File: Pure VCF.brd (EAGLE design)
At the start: 33.6 x 100 mm, 82 parts, among them T1 TRANS_PAIR_PNP, U1 QUAD_OPAMP, U2 LM13700, U3 DUAL_OPAMP, U4 LM13700

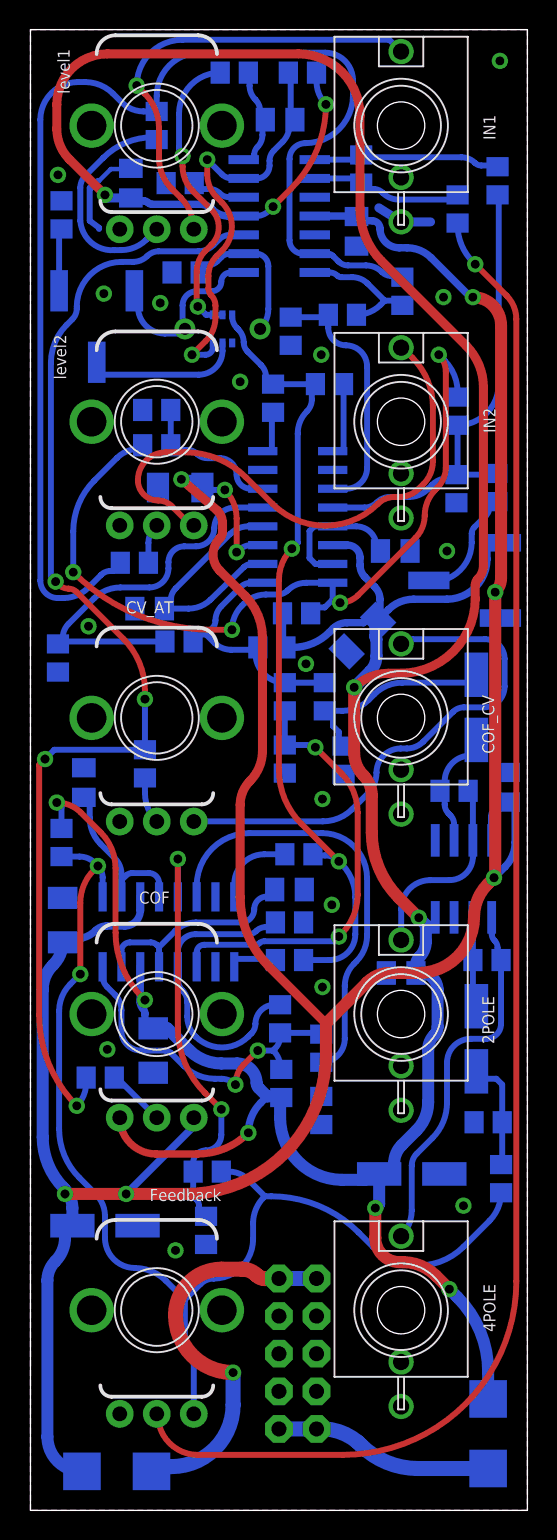
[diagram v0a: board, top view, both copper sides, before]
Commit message: VCF 2.2
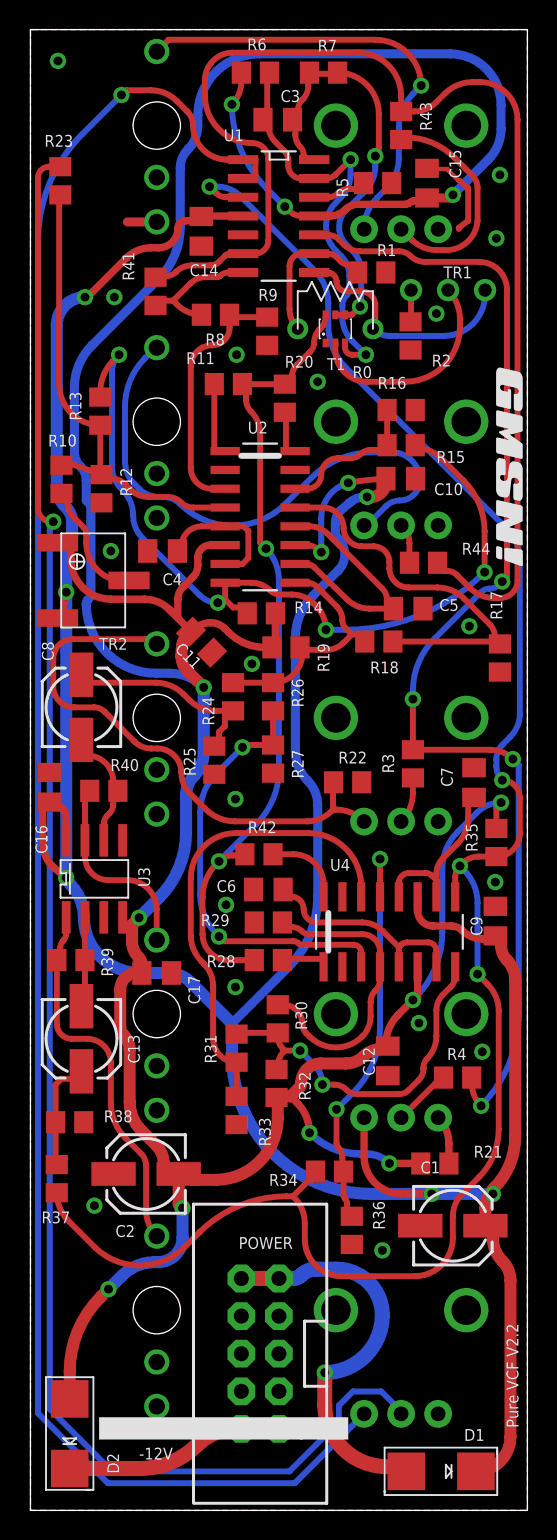
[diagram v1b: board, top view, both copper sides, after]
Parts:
- added U$1, U$2: (no value), gmsnLogo:GMSN!_LOGO
- C10, C11, C12, C9: value 100nF -> 0.1u; device rcl:C1206K -> rcl:C0805K
- C14, C15, C16, C17: value * -> 0.1u
- R21: value 300K -> 75K***
- R22: value 49K9 -> 1M***
- R23: value 100K -> 4k12
- R3: value 100K -> 1M***
- R39: value 2K2 -> 4k12
- R4: value 100K -> 1M5***
- R6: value 220K -> 2M***
- R7: value 2K2 -> 0R***
- TR1: value 100R -> 100K; device INSTRUO:TRIM_3269W -> INSTRUO:TRIMMER_TH3
- TR2: value 100R -> 100k
- moved R21 67.3 mm to (28.3, 40.2), flipped to the top, turned to 0 degrees
- moved R22 39.4 mm to (22.4, 65.9), flipped to the top, turned to 0 degrees
- moved C16 31.0 mm to (2.30, 65.6), flipped to the top
- moved R37 30.0 mm to (2.78, 39.1), flipped to the top
- moved R17 29.8 mm to (32.7, 74.3), flipped to the top
- moved R23 29.5 mm to (3.02, 106.5), flipped to the top
- moved R10 29.4 mm to (3.10, 86.4), flipped to the top
- moved R35 29.4 mm to (32.5, 61.8), flipped to the top
- moved C9 29.2 mm to (32.4, 56.5), flipped to the top
- moved D2 28.3 mm to (3.65, 21.9), flipped to the top
- moved R38 28.3 mm to (3.65, 42.9), flipped to the top
- moved R39 28.1 mm to (3.73, 53.9), flipped to the top
- moved C13 26.7 mm to (4.45, 48.6), flipped to the top
- moved C8 26.7 mm to (4.45, 71.0), flipped to the top
- moved C7 26.4 mm to (31.0, 65.9), flipped to the top
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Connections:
- net -12V: now also R21.1; no longer COF.P$1
- net GND: now also R22.2; no longer U1.1+IN
- net N$19: now also R23.1; no longer R22.1
- net N$20: now also Q.P$3, U1.1OUT; no longer R21.1, R22.2
- net N$25: now also COF.P$1; no longer R23.1, U1.1OUT
- net N$46: now also U1.1+IN; no longer Q.P$3
- net N$7: now also R22.1
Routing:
- net N$20: track 10.4 -> 129.9 mm, vias 0 -> 1
- net N$46: track 77.9 -> 125.9 mm, vias 2 -> 4
- net N$19: track 103.0 -> 114.6 mm
- net N$25: track 12.9 -> 3.24 mm
- net N$5: track 11.9 -> 15.8 mm
- net N$2: track 10.4 -> 14.0 mm
- net +12V: track 206.1 -> 209.2 mm
- net N$7: track 34.3 -> 36.5 mm
- net N$3: track 4.21 -> 2.18 mm
- net N$56: track 0.00 -> 1.91 mm
- net -12V: track 243.7 -> 241.8 mm, vias 10 -> 11
- net N$8: track 79.1 -> 80.9 mm
- net GND: track 10.3 -> 8.48 mm, vias 16 -> 18
- net N$44: track 23.4 -> 25.1 mm
- net N$40: track 28.6 -> 27.8 mm
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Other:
- board text added: "Pure VCF V2.2"
- board text added: "copyright GMSN Ltd 2016"
